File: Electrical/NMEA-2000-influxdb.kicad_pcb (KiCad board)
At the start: 4 copper layers, 149.9 x 70 mm, 32 parts, among them J1 Conn_01x04, J2 Conn_01x04, J3 Conn_01x02, J4 Micro_SD_Card, J5 Conn_02x08, U1 LM7805_TO220, U2 ESP32_NODEMCU, U3 SN65HVD230, U4 SN65HVD230-Module, U5 SD-Card-Module

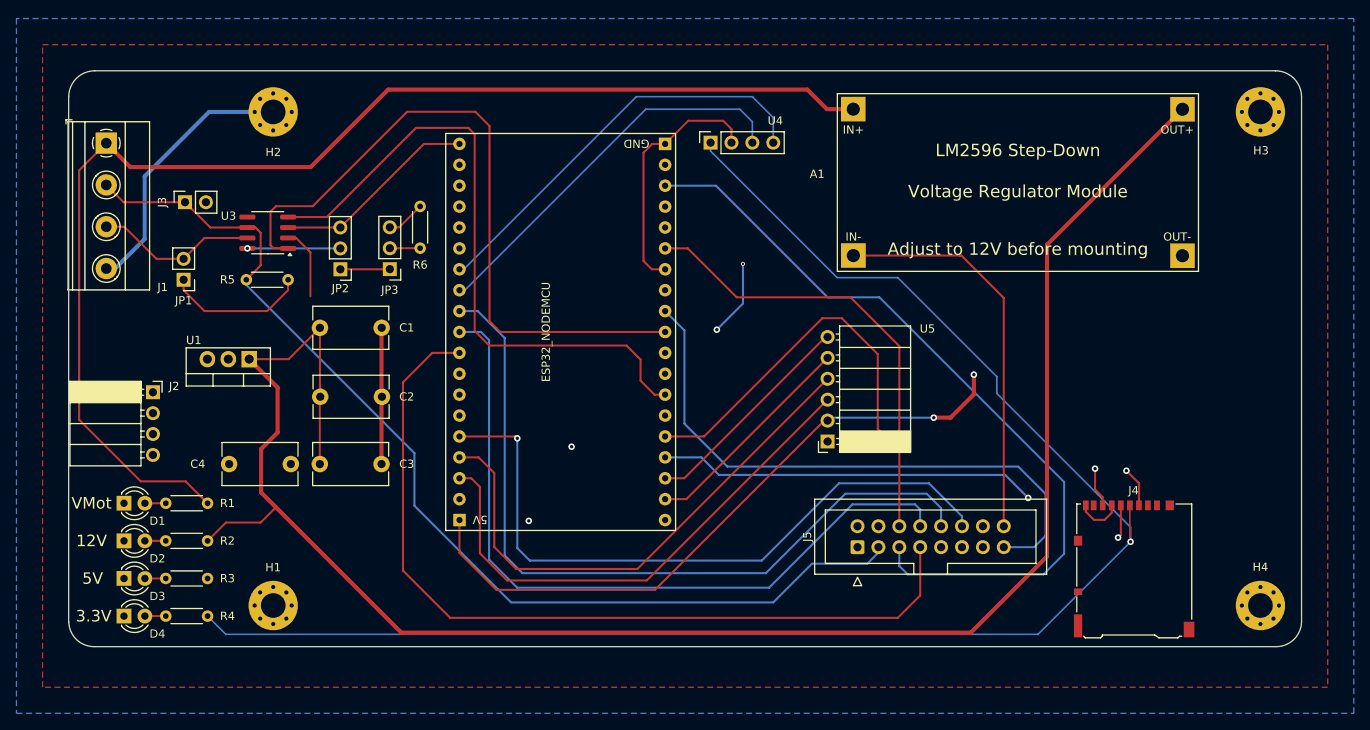
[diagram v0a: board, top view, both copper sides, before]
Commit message: Finished Rev 4 Schematics
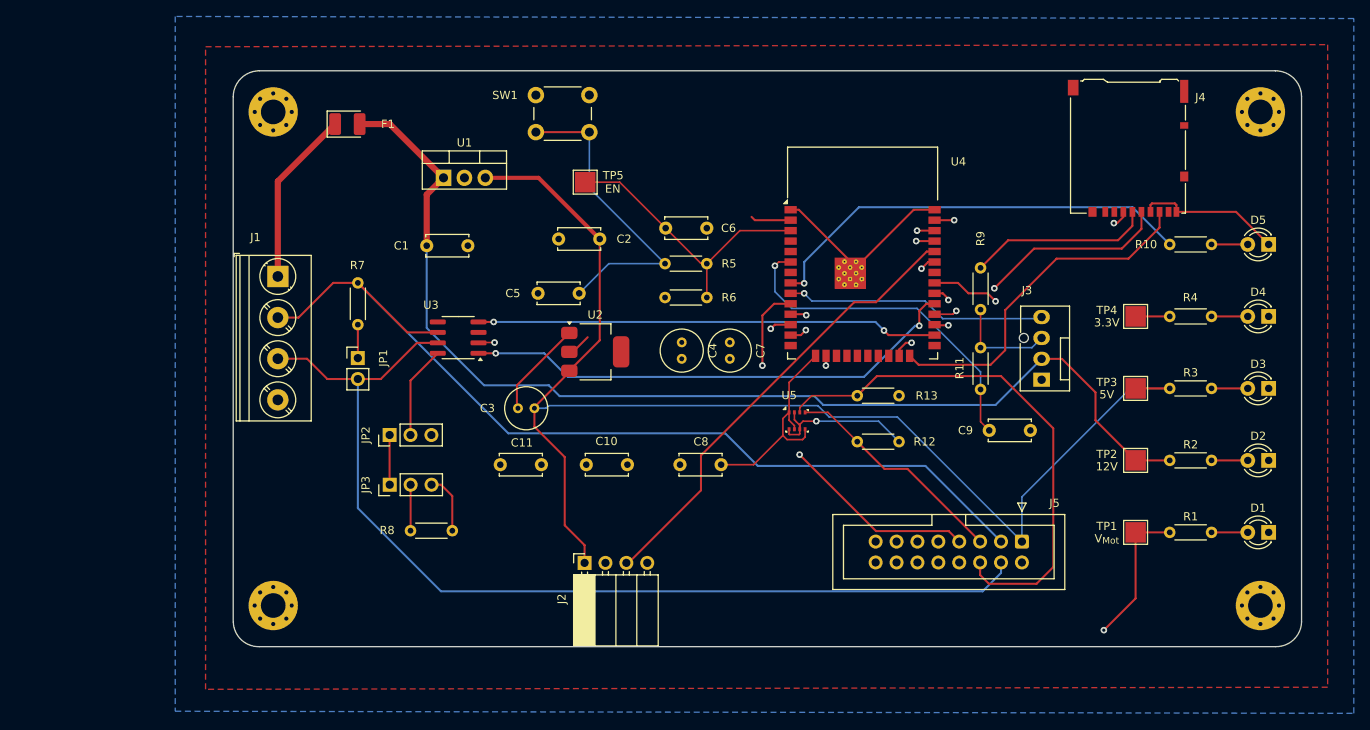
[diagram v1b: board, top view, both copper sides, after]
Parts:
- removed A1: LM2596_Step_Down_Module, LM2596:LM2596_Step_Down_Module-21.3x43.6mm
- added C10: 0.1uF, Capacitor_THT:C_Disc_D5.0mm_W2.5mm_P5.00mm, F.Cu at (142.5, 106.2)
- added C11: 0.1uF, Capacitor_THT:C_Disc_D5.0mm_W2.5mm_P5.00mm, F.Cu at (127.0, 106.2)
- added C5: 0.1uF, Capacitor_THT:C_Disc_D5.0mm_W2.5mm_P5.00mm, F.Cu at (131.6, 85.3)
- added C6: 1uF, Capacitor_THT:C_Disc_D5.0mm_W2.5mm_P5.00mm, F.Cu at (152.1, 77.4)
- added C7: 22uF, Capacitor_THT:C_Radial_D5.0mm_H7.0mm_P2.00mm, F.Cu at (154.9, 91.3)
- added C8: 0.1uF, Capacitor_THT:C_Disc_D5.0mm_W2.5mm_P5.00mm, F.Cu at (148.9, 106.2)
- added C9: 0.1nF, Capacitor_THT:C_Disc_D5.0mm_W2.5mm_P5.00mm, F.Cu at (186.5, 102.0)
- added D5: LED, LED_THT:LED_D3.0mm, F.Cu at (220.4, 79.4)
- added F1: Polyfuse, Diode_SMD:D_1210_3225Metric_Pad1.42x2.65mm_HandSolder, F.Cu at (108.5, 64.8)
- added R10: 330R, Resistor_THT:R_Axial_DIN0204_L3.6mm_D1.6mm_P5.08mm_Horizontal, F.Cu at (208.4, 79.4)
- added R11: 3.3k, Resistor_THT:R_Axial_DIN0204_L3.6mm_D1.6mm_P5.08mm_Horizontal, F.Cu at (185.4, 97.0)
- added R12: 4.7k, Resistor_THT:R_Axial_DIN0204_L3.6mm_D1.6mm_P5.08mm_Horizontal, F.Cu at (170.4, 103.4)
- added R13: 4.7k, Resistor_THT:R_Axial_DIN0204_L3.6mm_D1.6mm_P5.08mm_Horizontal, F.Cu at (170.4, 97.8)
- added R7: 120R, Resistor_THT:R_Axial_DIN0204_L3.6mm_D1.6mm_P5.08mm_Horizontal, F.Cu at (109.7, 89.2)
- added R8: 10k, Resistor_THT:R_Axial_DIN0204_L3.6mm_D1.6mm_P5.08mm_Horizontal, F.Cu at (121.2, 114.2)
- added R9: 10k, Resistor_THT:R_Axial_DIN0204_L3.6mm_D1.6mm_P5.08mm_Horizontal, F.Cu at (185.4, 82.2)
- added SW1: SW_Push, Button_Switch_THT:SW_PUSH_6mm, F.Cu at (131.4, 61.2)
- added TP1: V_{Mot}, TestPoint:TestPoint_Pad_2.5x2.5mm, F.Cu at (204.3, 114.4)
- added TP2: 12V, TestPoint:TestPoint_Pad_2.5x2.5mm, F.Cu at (204.3, 105.7)
- added TP3: 5V, TestPoint:TestPoint_Pad_2.5x2.5mm, F.Cu at (204.3, 96.9)
- added TP4: 3.3V, TestPoint:TestPoint_Pad_2.5x2.5mm, F.Cu at (204.3, 88.2)
- added TP5: EN, TestPoint:TestPoint_Pad_2.5x2.5mm, F.Cu at (137.4, 71.8)
- C1: value 0.1uF -> 0.33uF; footprint Capacitor_THT:C_Disc_D9.0mm_W5.0mm_P7.50mm -> Capacitor_THT:C_Disc_D5.0mm_W2.5mm_P5.00mm
- C2: footprint Capacitor_THT:C_Disc_D9.0mm_W5.0mm_P7.50mm -> Capacitor_THT:C_Disc_D5.0mm_W2.5mm_P5.00mm
- C3, C4: value 0.1uF -> 22uF; footprint Capacitor_THT:C_Disc_D9.0mm_W5.0mm_P7.50mm -> Capacitor_THT:C_Radial_D5.0mm_H7.0mm_P2.00mm
- J1: footprint TerminalBlock_Phoenix:TerminalBlock_Phoenix_MKDS-1,5-4-5.08_1x04_P5.08mm_Horizontal -> TerminalBlock_Phoenix:TerminalBlock_Phoenix_PT-1,5-4-5.0-H_1x04_P5.00mm_Horizontal
- J3: value Conn_01x02 -> Conn_01x04; footprint Connector_PinSocket_2.54mm:PinSocket_1x02_P2.54mm_Vertical -> Connector:FanPinHeader_1x04_P2.54mm_Vertical
- R5: value 120R -> 0R
- U2: value ESP32_NODEMCU -> AMS1117-3.3; footprint esp32:esp32 -> Package_TO_SOT_SMD:SOT-223-3_TabPin2
- U4: value SN65HVD230-Module -> ESP32-WROOM-32E; footprint Connector_PinSocket_2.54mm:PinSocket_1x04_P2.54mm_Vertical -> RF_Module:ESP32-WROOM-32D
- U5: value SD-Card-Module -> BME280; footprint Connector_PinSocket_2.54mm:PinSocket_1x06_P2.54mm_Horizontal -> Package_LGA:Bosch_LGA-8_2.5x2.5mm_P0.65mm_ClockwisePinNumbering
- moved D4 143.8 mm to (220.4, 88.2), turned to 180 degrees
- moved D3 141.0 mm to (220.4, 96.9), turned to 180 degrees
- moved D2 139.5 mm to (220.4, 105.7), turned to 180 degrees
- moved D1 139.2 mm to (220.4, 114.4), turned to 180 degrees
- moved H3 134.2 mm to (99.4, 123.3)
- moved R4 122.5 mm to (208.4, 88.2), turned to 0 degrees
- moved H2 120.0 mm to (219.4, 63.3)
- moved R3 119.2 mm to (208.4, 96.9), turned to 0 degrees
- moved R2 117.4 mm to (208.4, 105.7), turned to 0 degrees
- moved R1 117.0 mm to (208.4, 114.4), turned to 0 degrees
- moved J3 106.3 mm to (192.8, 95.8)
- moved H1 60.0 mm to (99.4, 63.3)
- moved C4 57.0 mm to (149.1, 91.3), turned to -90 degrees
- moved J2 56.4 mm to (137.3, 118.1), turned to 90 degrees
- moved J4 51.1 mm to (203.4, 67.7), turned to 180 degrees
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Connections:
- C2 pad 1: +12V -> +5V
- C3 pad 1: +12V -> +5V
- C4 pad 1: +5V -> +3.3V
- J2 pad 2: /RX -> /TX
- J2 pad 3: /TX -> /RX
- J3 pad 1: /CAN_H -> GND
- J3 pad 2: /CAN_L -> +12V
- J4 pad 4: +3V3 -> +3.3V
- J5 pad 2: +3V3 -> +3.3V
- JP2 pad 3: +3V3 -> +3.3V
- R4 pad 1: +3V3 -> +3.3V
- R5 pad 1: Net-(JP1-A) -> Net-(C5-Pad2)
- R5 pad 2: /CAN_H -> /EN
- R6 pad 1: GND -> /EN
- R6 pad 2: Net-(JP3-C) -> +3.3V
- U2 pad 1: +5V -> GND
- U2 pad 2: unconnected-(U2-CMD-Pad2) -> +3.3V
- U2 pad 3: /MISO -> +5V
- U3 pad 3: +3V3 -> +3.3V
- U4 pad 1: +3V3 -> GND
- U4 pad 2: GND -> +3.3V
- U4 pad 3: /CAN_RX_B -> /EN
- U4 pad 4: /CAN_TX_B -> unconnected-(U4-SENSOR_VP-Pad4)
- U5 pad 2: +5V -> +3.3V
- U5 pad 3: /MISO -> /SDA
- U5 pad 4: /MOSI -> /SCL
- U5 pad 5: /SCK -> GND
- U5 pad 6: /CS -> +3.3V
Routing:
- net +3V3: track 319.5 -> 0.00 mm, vias 1 -> 0
- net GND: track 215.2 -> 90.3 mm, vias 3 -> 1
- net +12V: track 222.8 -> 135.6 mm
- net /MOSI: track 65.2 -> 0.00 mm
- net /MISO: track 63.7 -> 0.00 mm
- net /SW_TG: track 103.5 -> 43.2 mm, vias 0 -> 2
- net /CLK: track 107.1 -> 50.1 mm, vias 1 -> 2
- net /TX: track 119.7 -> 65.7 mm, vias 0 -> 1
- net Net-(U4-IO32): track 0.00 -> 53.3 mm, vias 0 -> 1
- net +3.3V: track 0.00 -> 53.0 mm, vias 0 -> 1
- net /GREEN: track 103.9 -> 51.1 mm, vias 0 -> 1
- net /CAN_TX_B: track 50.9 -> 0.00 mm
- net /RX: track 104.6 -> 55.6 mm
- net /CAN_RX_B: track 47.9 -> 0.00 mm
- net +5V: track 115.0 -> 161.4 mm, vias 3 -> 0
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- added copper zone on F.Cu, net +3.3V
- added copper zone on B.Cu, net GND
- removed copper zone on B.Cu, net +5V
- removed copper zone on F.Cu, net GND
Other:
- board size 149.9 x 70 mm -> 129.9 x 70 mm
